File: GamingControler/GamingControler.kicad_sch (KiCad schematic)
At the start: 52 parts, among them J1 USB_C_Receptacle_USB2.0_16P, J2 USB_C_Receptacle_USB2.0_16P, J3 Conn_01x05_Pin, J4 Conn_01x05_Pin, SW1 SW_Push, SW2 SW_Push, U1 ESP32-C6-WROOM-1, U2 AZ1117-3.3, U3 CP2102N-Axx-xQFN20, U4 TTP223-BA6, U5 TTP223-BA6, U6 TTP223-BA6, U7 TTP223-BA6

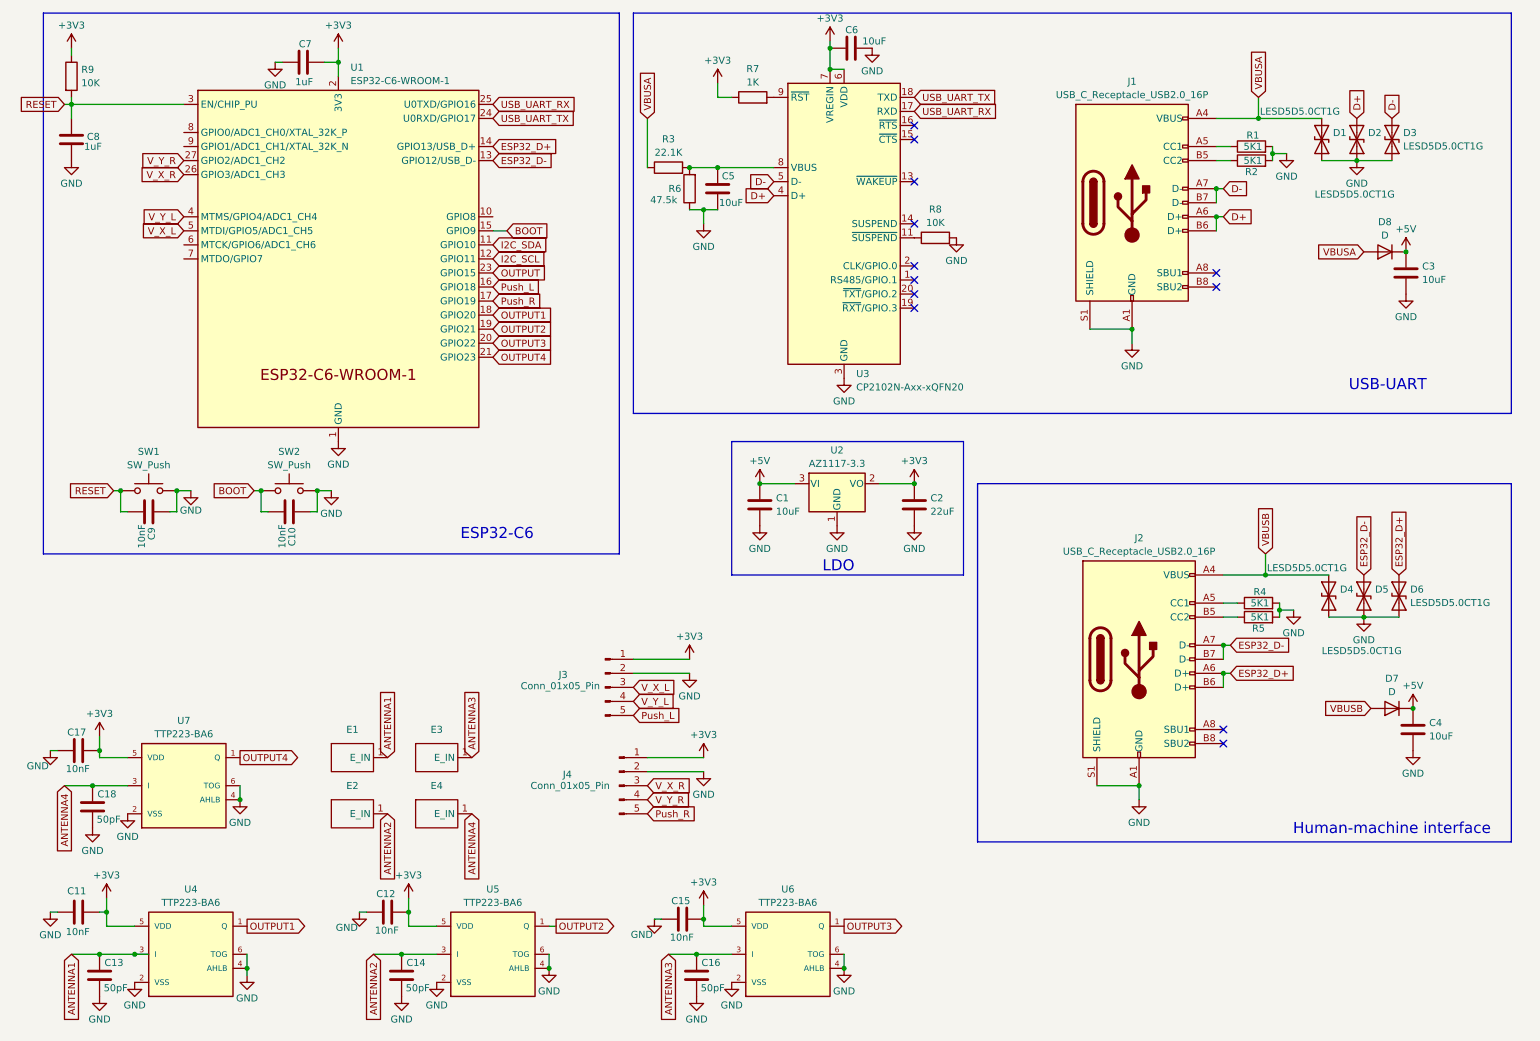
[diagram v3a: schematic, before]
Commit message: Gaming controller
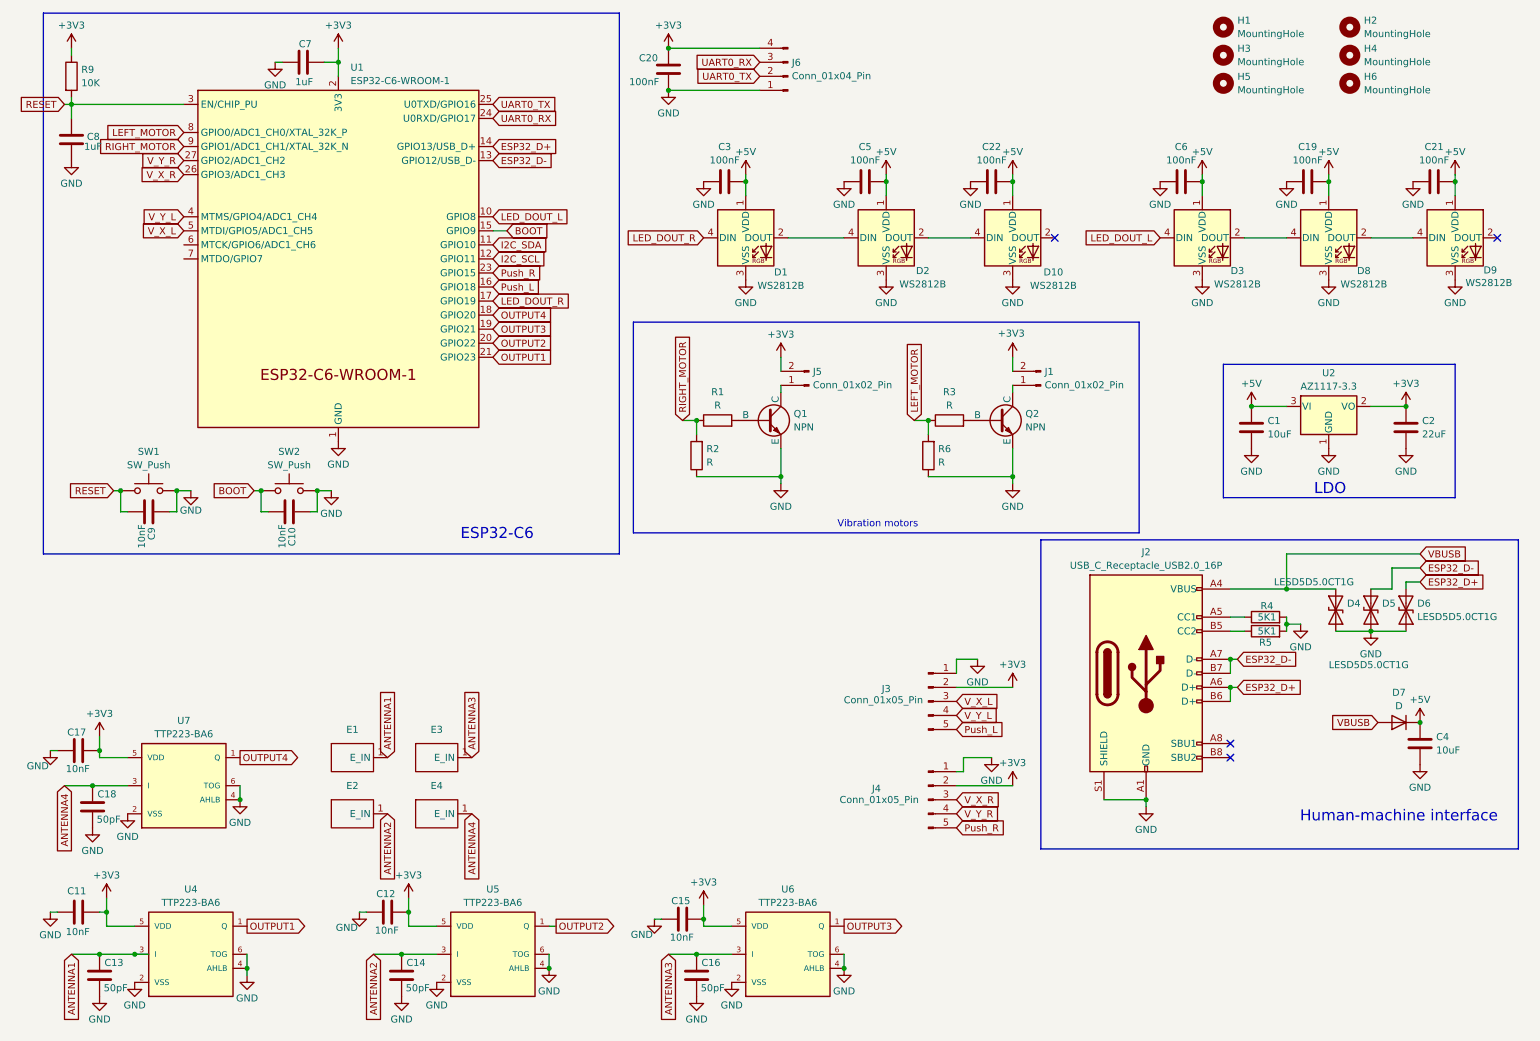
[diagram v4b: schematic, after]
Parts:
- removed D1, D2, D3: LESD5D5.0CT1G, Diode_SMD:D_SOD-523, symbol Diode:1.5KExxCA
- removed D8: D, Diode_SMD:D_0805_2012Metric, symbol Device:D
- removed J1: USB_C_Receptacle_USB2.0_16P, Connector_USB:USB_C_Receptacle_G-Switch_GT-USB-7010ASV, symbol Connector:USB_C_Receptacle_USB2.0_16P
- removed R7: 1K, Resistor_SMD:R_0805_2012Metric, symbol Device:R
- removed R8: 10K, Resistor_SMD:R_0805_2012Metric, symbol Device:R
- removed U3: CP2102N-Axx-xQFN20, Package_DFN_QFN:SiliconLabs_QFN-20-1EP_3x3mm_P0.5mm_EP1.8x1.8mm_ThermalVias, symbol Interface_USB:CP2102N-Axx-xQFN20
- added C19, C20, C21, C22: 100nF, Capacitor_SMD:C_0805_2012Metric, symbol Device:C
- added D1, D10, D2, D3, D8, D9: WS2812B, LED_SMD:LED_WS2812B_PLCC4_5.0x5.0mm_P3.2mm, symbol LED:WS2812B
- added H1, H2, H3, H4, H5, H6: MountingHole, MountingHole:MountingHole_3.2mm_M3, symbol Mechanical:MountingHole
- added J1, J5: Conn_01x02_Pin, Connector_PinSocket_2.00mm:PinSocket_1x02_P2.00mm_Vertical, symbol Connector:Conn_01x02_Pin
- added J6: Conn_01x04_Pin, Connector_PinSocket_2.54mm:PinSocket_1x04_P2.54mm_Vertical, symbol Connector:Conn_01x04_Pin
- added Q1, Q2: NPN, Package_TO_SOT_SMD:SOT-23, symbol Simulation_SPICE:NPN
- C3, C5, C6: value 10uF -> 100nF
- R1, R2: value 5K1 -> R
- R3: value 22.1K -> R
- R6: value 47.5k -> R
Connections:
- net OUTPUT is gone; now on net Push_R: U1.23 (GPIO15)
- net VBUSA is gone; now on net LEFT_MOTOR: R3.1
- net +3V3: now also J3.2 (Pin_2), J4.2 (Pin_2), C20.2, J1.2 (Pin_2), J5.2 (Pin_2), J6.4 (Pin_4); no longer C6.1, J3.1 (Pin_1), J4.1 (Pin_1)
- net +5V: now also C3.2, C5.2, C6.2, C19.2, C21.2, C22.2, D1.1 (VDD), D10.1 (VDD), D2.1 (VDD), D3.1 (VDD), D8.1 (VDD), D9.1 (VDD); no longer C3.1
- net GND: now also C3.1, C5.1, C6.1, J3.1 (Pin_1), J4.1 (Pin_1), R2.1, C19.1, C20.1, C21.1, C22.1, D1.3 (VSS), D10.3 (VSS), D2.3 (VSS), D3.3 (VSS), D8.3 (VSS), D9.3 (VSS), J6.1 (Pin_1), Q1.3 (E), Q2.3 (E); no longer C3.2, C5.2, C6.2, J3.2 (Pin_2), J4.2 (Pin_2), R1.2, R2.2
- net OUTPUT1: now also U1.21 (GPIO23); no longer U1.18 (GPIO20)
- net OUTPUT2: now also U1.20 (GPIO22); no longer U1.19 (GPIO21)
- net OUTPUT3: now also U1.19 (GPIO21); no longer U1.20 (GPIO22)
- net OUTPUT4: now also U1.18 (GPIO20); no longer U1.21 (GPIO23)
- net Push_R: no longer U1.17 (GPIO19)
- net RIGHT_MOTOR: now reaches R1.1
- net RIGHT_MOTOR: now also R2.2, U1.9 (GPIO1/ADC1_CH1/XTAL_32K_N)
- net LED_DOUT_L: now reaches U1.10 (GPIO8)
- net LED_DOUT_L: now also D3.4 (DIN)
- net LEFT_MOTOR: now reaches U1.8 (GPIO0/ADC1_CH0/XTAL_32K_P)
- net LEFT_MOTOR: now also R6.2
- net USB_UART_RX renamed UART0_TX
- net UART0_TX: now also J6.2 (Pin_2)
- net USB_UART_TX renamed UART0_RX
- net UART0_RX: now also J6.3 (Pin_3)
- new net: Q1.2 (B), R1.2
- new net: D10.4 (DIN), D2.2 (DOUT)
- new net: J1.1 (Pin_1), Q2.1 (C)
- new net: Q2.2 (B), R3.2
- new net: D1.2 (DOUT), D2.4 (DIN)
- new net: D8.2 (DOUT), D9.4 (DIN)
- new net: J5.1 (Pin_1), Q1.1 (C)
- new net: D3.2 (DOUT), D8.4 (DIN)
- new net LED_DOUT_R: D1.4 (DIN), U1.17 (GPIO19)
- no-connect marks 12 -> 4
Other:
- note added: "Vibration motors"
- note removed: "USB-UART"
- moved on the sheet: C1, C2, C4, D4, D5, D6, D7, J2, J3, J4, R4, R5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
